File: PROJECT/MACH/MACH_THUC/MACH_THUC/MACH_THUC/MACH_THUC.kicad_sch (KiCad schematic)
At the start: 66 parts, among them K1 SANYOU_SRD_Form_C, K2 SANYOU_SRD_Form_C, Q1 2SB688, Q2 BC547, Q3 BC547, U1 LM7805_TO220, U2 DS1307+, U3 LCD-016N002L, U4 PCF8574, U5 PC817, U6 PC817, Y1 Crystal 20M, Y2 Crystal 32.768KHz

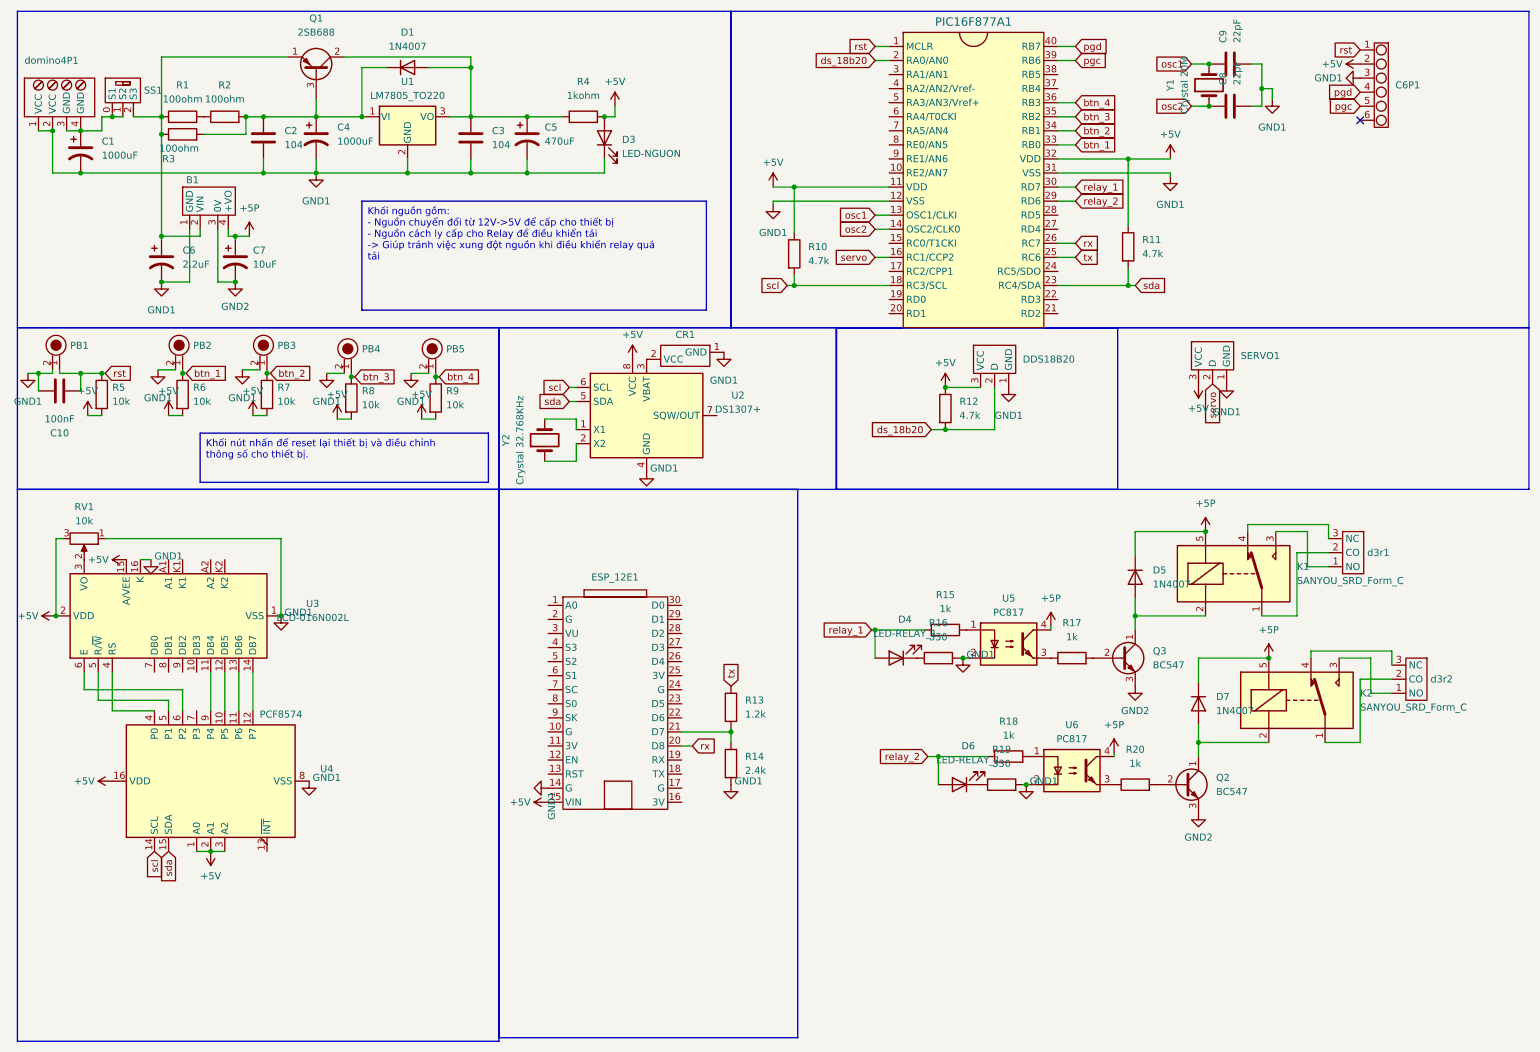
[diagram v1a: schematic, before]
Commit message: update for finnal code
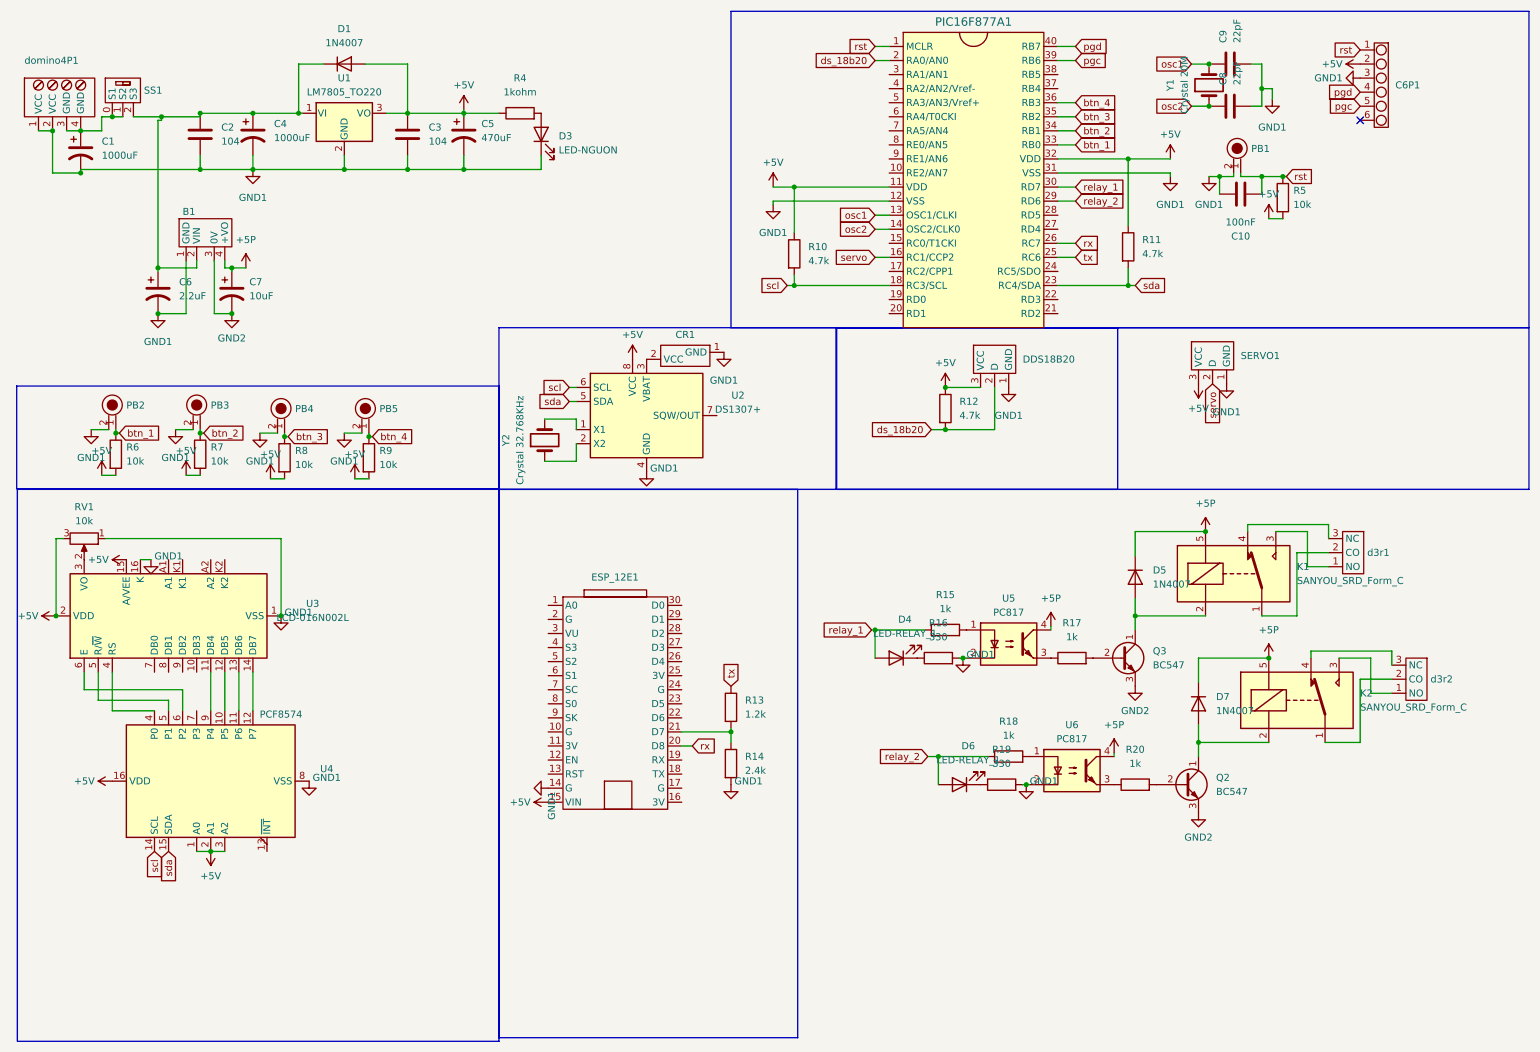
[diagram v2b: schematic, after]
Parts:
- removed Q1: 2SB688, Package_TO_SOT_THT:TO-218-3_Vertical, symbol Transistor_BJT:2SB631
- removed R1, R2, R3: 100ohm, library_thuan_footprint:RES_1ohm_1w, symbol Device:R
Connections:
- net +5V: now also C3.1, C5.1, D1.2 (A), R4.1, U1.3 (VO); no longer D3.2 (A), R4.2
- net at B1.2 (VIN), C6.1, SS1.2 (S3): now also C2.1, C4.1, D1.1 (K), U1.1 (VI)
- new net: D3.2 (A), R4.2
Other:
- moved on the sheet: B1, C10, C2, C3, C4, C5, C6, C7, D1, D3, PB1, PB2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
